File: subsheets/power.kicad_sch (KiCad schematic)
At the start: 48 parts, among them P1 USB_C_Plug, U1 CP2102N-Axx-xQFN24, U2 MCP73871_U, U3 LP2985-3.3

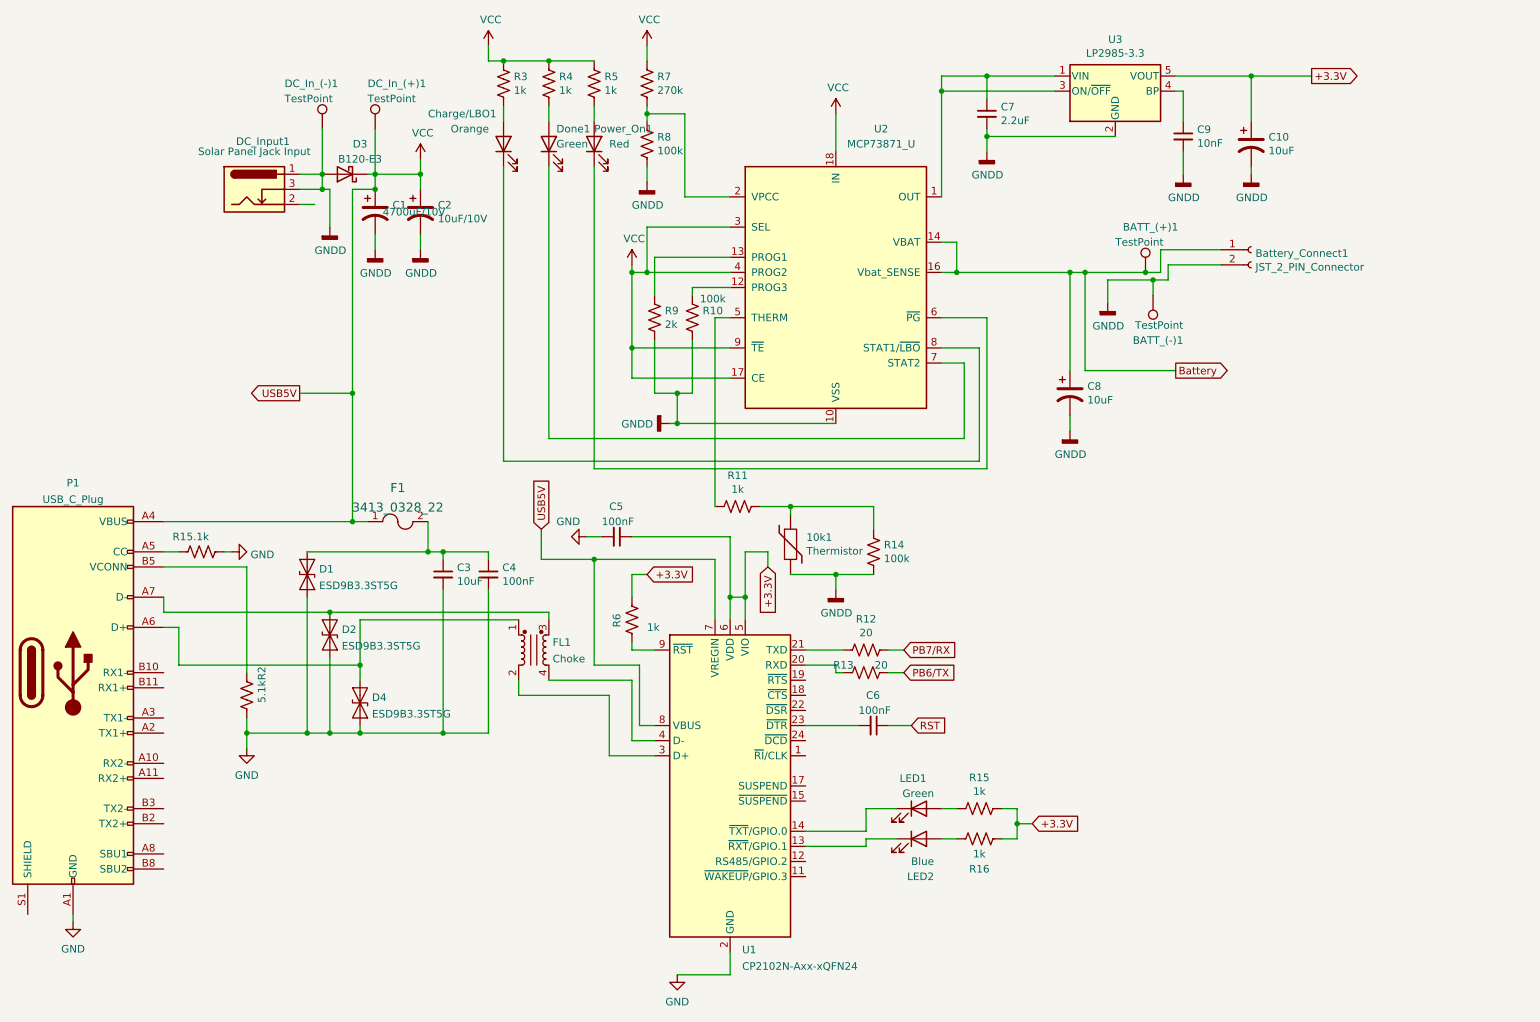
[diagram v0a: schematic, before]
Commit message: A few schematic changes and fixes
-
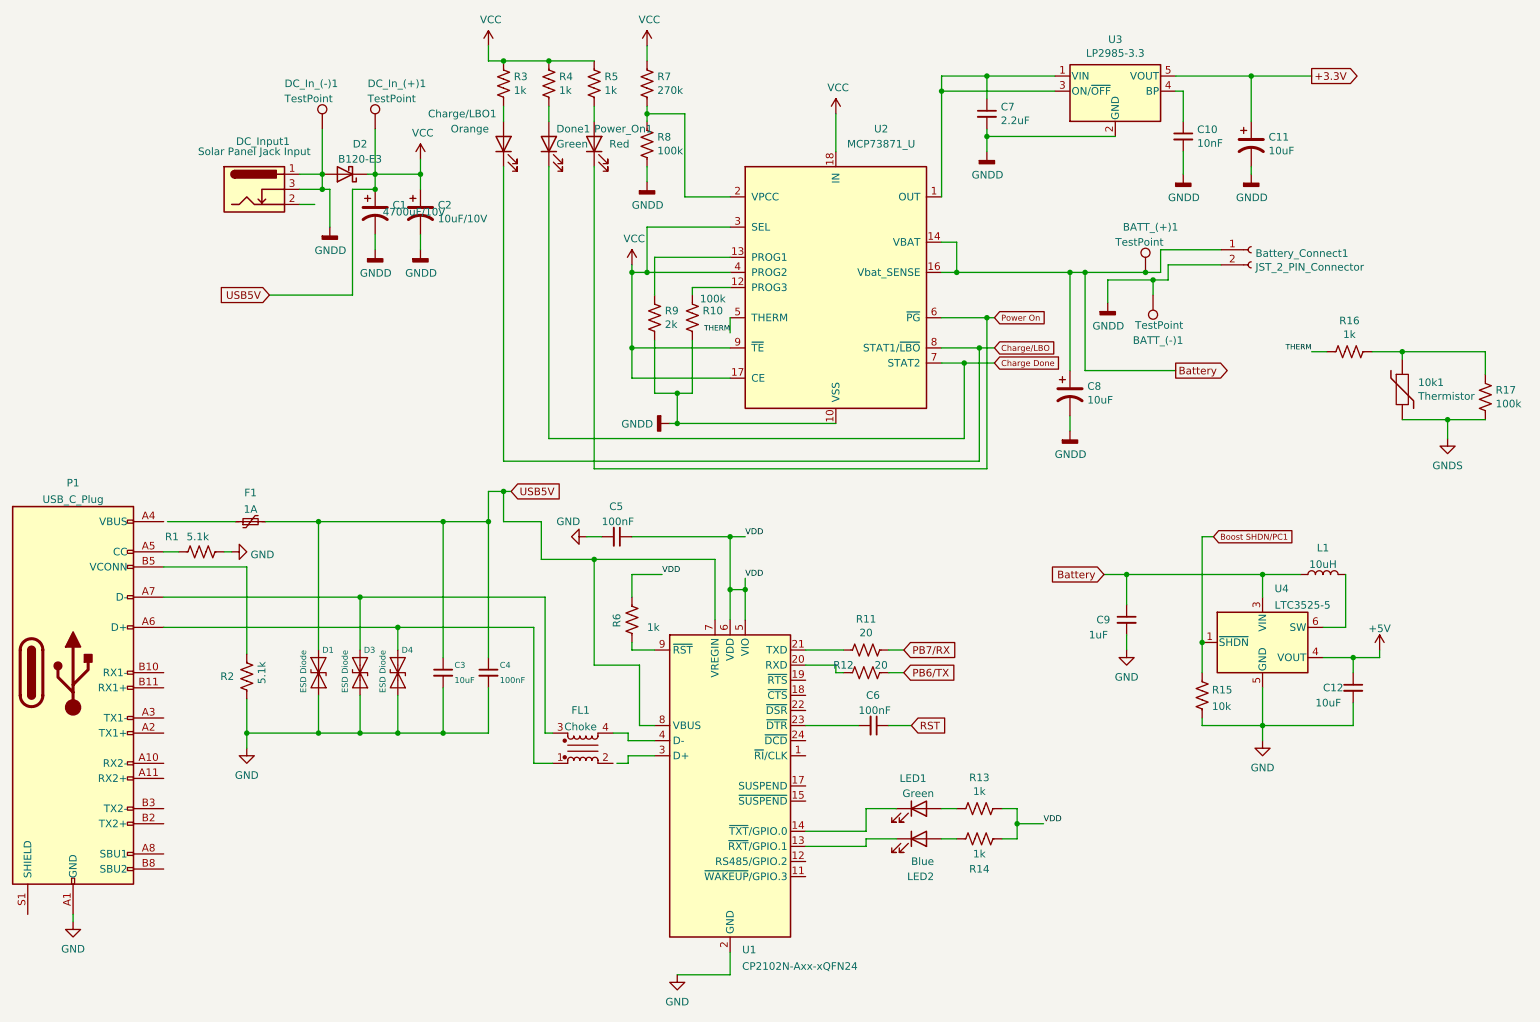
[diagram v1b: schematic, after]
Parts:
- removed F1: 3413_0328_22, digikey-footprints:1206, symbol dk_Fuses:3413_0328_22
- added C12: 10uF, symbol Device:C_Small
- added C9: 1uF, symbol Device:C_Small
- added F1: 1A, symbol Device:Polyfuse_Small
- added L1: 10uH, symbol Device:L
- added R15: 10k, symbol Device:R_US
- added U4: LTC3525-5, Package_TO_SOT_SMD:SOT-363_SC-70-6, symbol Regulator_Switching:LTC3525-5
- D1, D4: value ESD9B3.3ST5G -> ESD Diode
- D3: renamed from D2; value ESD9B3.3ST5G -> ESD Diode
- renumbered C9 to C10, C10 to C11, D3 to D2, R12 to R11, R13 to R12, R15 to R13, R16 to R14, R11 to R16, R14 to R17
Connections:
- net +3.3V: no longer C5.1, R13.1, R14.1, R6.2, U1.5 (VIO), U1.6 (VDD)
- net Battery: now also C9.1, L1.1, U4.3 (VIN)
- net GND: now also C12.2, C9.2, R15.2, U4.2 (GND), U4.5 (GND)
- net GNDD: no longer 10k1.2, R17.1
- net VCC: now also C3.1, C4.1, D1.1 (A1), F1.2; no longer P1.A4 (VBUS), P1.A9 (VBUS), P1.B4 (VBUS), P1.B9 (VBUS)
- net THERM: now reaches R16.2, U2.5 (THERM)
- net Power On: now reaches Power_On1.1 (K), U2.6 (~{PG})
- net Charge Done: now reaches Done1.1 (K), U2.7 (STAT2)
- net Charge/LBO : now reaches Charge/LBO1.1 (K), U2.8 (STAT1/~{LBO})
- net at U1.3 (D+): no longer FL1.2
- new net: P1.A4 (VBUS), P1.A9 (VBUS), P1.B4 (VBUS), P1.B9 (VBUS)
- new net: L1.2, U4.6 (SW)
- new net +5V: C12.1, U4.4 (VOUT)
- new net Boost SHDN/PC1: R15.1, U4.1 (~{SHDN})
- new net GNDS: 10k1.2, R17.1
- new net VDD: C5.1, R13.1, R14.1, R6.2, U1.5 (VIO), U1.6 (VDD)
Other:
- moved on the sheet: 10k1, C3, C4, D1, D3, D4, FL1, R16, R17, R2
